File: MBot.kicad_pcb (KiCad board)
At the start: 4 copper layers, 50 x 55 mm, 111 parts, among them J1 Micro_SD_Card_Det1, J10 Conn_01x04, J11 Conn_01x06, J12 Conn_01x04, J14 Conn_01x04, J16 Conn_01x06, J2 Barrel_Jack_Switch_Pin3Ring, J3 Screw_Terminal_01x02, J4 Conn_01x03, J5 Conn_01x06, J6 Conn_01x06, J7 Conn_01x06, J8 Conn_01x04, J9 Conn_01x04, SW1 SW_SPDT, SW2 SW_SPDT, SW3 SW_SPDT, SW4 SW_SPST, U1 74AUC1G19, U2 XL4015, U3 FM24W256

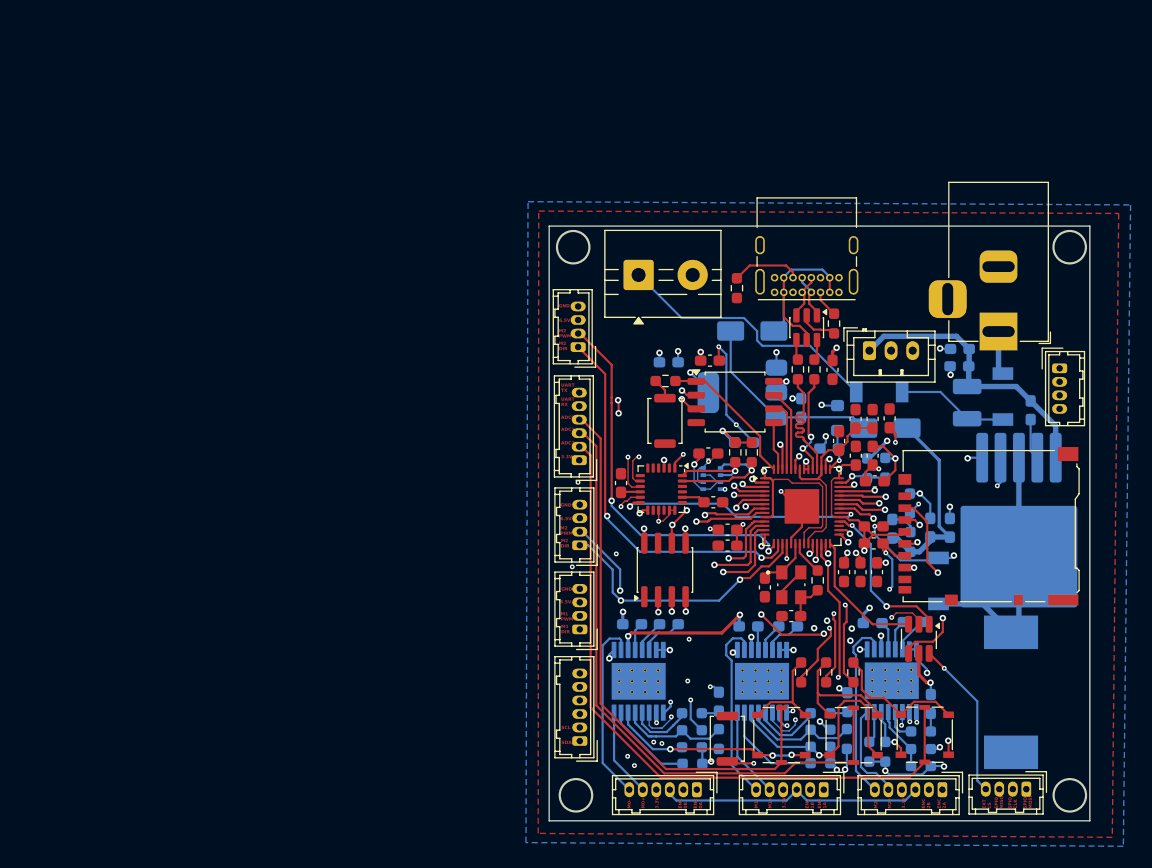
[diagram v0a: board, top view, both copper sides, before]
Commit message: Add files via upload
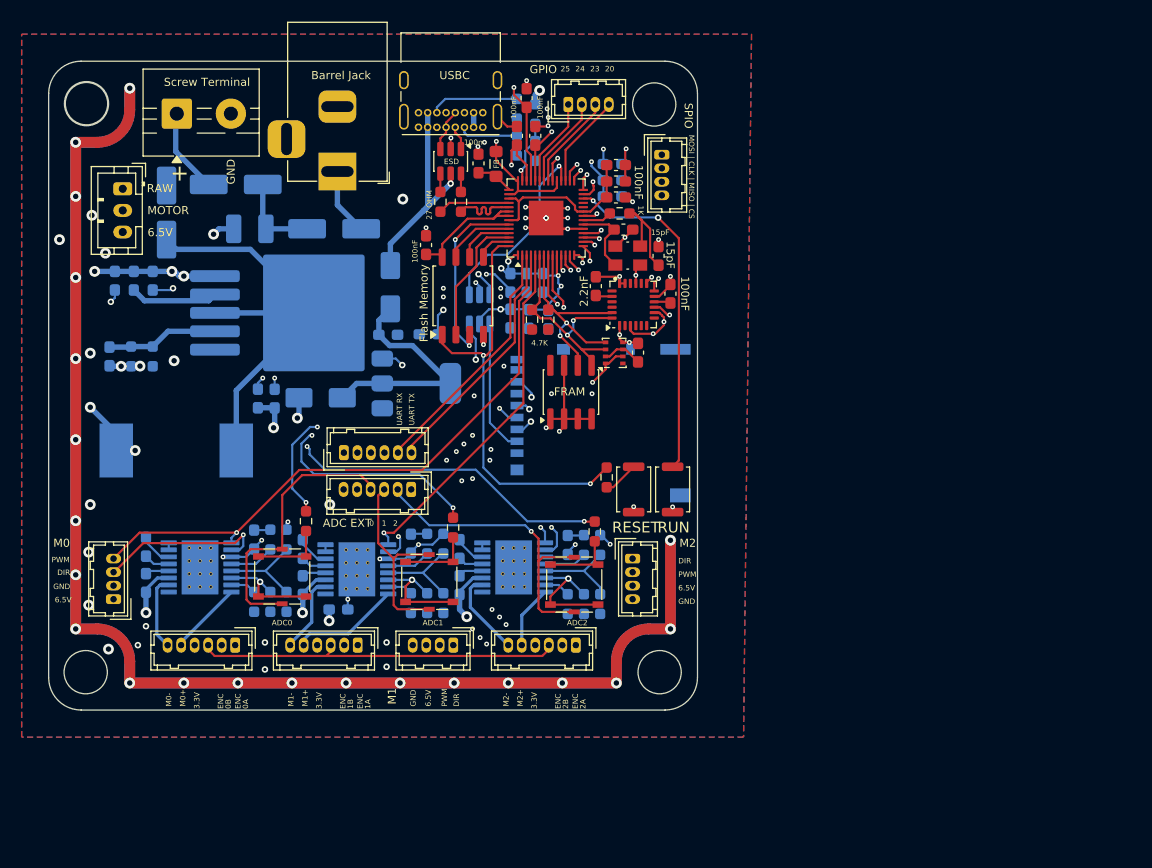
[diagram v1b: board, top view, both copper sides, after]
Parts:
- C109, C110, C111, C112, C113, C114, C115, C16, C17, J1, R109, RUSB1, U1: moved to B.Cu
- C120, FB1, UBarometer1: moved to F.Cu
- D4, D5, D6: value SS54FSH -> D; footprint SS54FSH:SODFL4725X110N -> Diode_SMD:D_SMA_Handsoldering
- moved CC1 83.8 mm to (67.9, 80.3)
- moved L1 80.4 mm to (71.8, 96.0), turned to 180 degrees
- moved D6 79.1 mm to (70.9, 74.0)
- moved C1 78.4 mm to (66.1, 80.3), turned to -90 degrees
- moved Cin1 75.0 mm to (69.6, 80.3), turned to -90 degrees
- moved CFF1 74.1 mm to (65.6, 87.3)
- moved R902 74.1 mm to (67.6, 87.3)
- moved R901 71.3 mm to (69.6, 87.3), turned to -90 degrees
- moved J4 70.7 mm to (66.8, 71.8), turned to -90 degrees
- moved U2 69.9 mm to (83.0, 83.3), turned to 0 degrees
- moved F1 68.3 mm to (78.6, 75.5), turned to 0 degrees
- moved J14 67.7 mm to (116.7, 68.7), turned to -90 degrees
- moved C18 65.1 mm to (79.3, 91.2)
- moved D4 63.8 mm to (86.4, 75.5), turned to 0 degrees
- moved J2 62.9 mm to (86.7, 70.2)
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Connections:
- F1 pad 2: Net-(D4-PadC) -> Net-(D4-K)
- J10 pad 1: M2_DIR -> M2_PWM
- J10 pad 2: M2_PWM -> M2_DIR
- J11 pad 5: UART0_RX -> unconnected-(J11-Pin_5-Pad5)
- J11 pad 6: UART0_TX -> unconnected-(J11-Pin_6-Pad6)
- J12 pad 1: unconnected-(J12-Pin_1-Pad1) -> GPIO25
- J12 pad 2: GPIO25 -> GPIO24
- J12 pad 3: GPIO24 -> GPIO23
- J12 pad 4: GPIO23 -> GPIO20
- J16 pad 5: unconnected-(J16-Pin_5-Pad5) -> UART0_RX
- J16 pad 6: unconnected-(J16-Pin_6-Pad6) -> UART0_TX
- J2 pad 1: Net-(D4-PadA) -> Net-(D4-A)
- J3 pad 1: Net-(J3-Pin_1) -> Net-(D5-A)
- J5 pad 1: ENC0A -> ENC0B
- J5 pad 2: ENC0B -> ENC0A
- J6 pad 1: ENC1A -> ENC1B
- J6 pad 2: ENC1B -> ENC1A
- J7 pad 1: ENC2A -> ENC2B
- J7 pad 2: ENC2B -> ENC2A
- J8 pad 1: M0_DIR -> +6V5
- J8 pad 2: M0_PWM -> GND
- J8 pad 3: +6V5 -> M0_DIR
- J8 pad 4: GND -> M0_PWM
- L1 pad 1: Net-(U2-SW) -> Net-(D6-K)
- U2 pad 3: Net-(U2-SW) -> Net-(D6-K)
- UDRV1 pad 27: GND -> (no net)
- UDRV1 pad 28: GND -> (no net)
- UDRV1 pad 29: GND -> (no net)
- ULDO1 pad 2: +3V3 -> Net-(D101-K)
- ULDO1 pad 3: Net-(D101-K) -> +3V3
- URP2040 pad 31: /RP2040/GPIO20 -> GPIO20
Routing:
- net GND: track 150.1 -> 337.6 mm, vias 46 -> 67
- net +6V5: track 18.2 -> 138.5 mm, vias 0 -> 10
- net VMOT: track 22.7 -> 126.4 mm, vias 8 -> 13
- net ADC1: track 24.8 -> 73.8 mm
- net ADC2: track 22.2 -> 69.8 mm
- net Net-(D6-K): track 0.00 -> 41.3 mm
- net ADC1_EXT: track 57.9 -> 18.4 mm
- net ADC2_EXT: track 63.9 -> 28.5 mm, vias 0 -> 1
- net ADC0: track 26.5 -> 57.1 mm
- net +3V3: track 103.2 -> 132.0 mm, vias 30 -> 39
- net /RP2040/QSPI_SS: track 13.5 -> 39.9 mm, vias 0 -> 2
- net ADC0_EXT: track 51.8 -> 25.9 mm
- net Net-(J3-Pin_1): track 25.1 -> 0.00 mm
- net Net-(U2-SW): track 24.2 -> 0.00 mm
- net M0_DIR: track 38.4 -> 61.5 mm, vias 3 -> 2
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- added copper zone on F.Cu, net +3V3
- added copper zone on In2.Cu, net +6V5
- added copper zone on In2.Cu, net BATT
- added copper zone on B.Cu, net GND
- added copper zone on In1.Cu, net GND
- removed copper zone on In1.Cu, net +3V3
- removed copper zone on B.Cu, net +6V5
- removed copper zone on F.Cu, net GND
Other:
- board size 50 x 55 mm -> 60 x 60 mm
- board text added: "+"
- board text added: "0"
- board text added: "0A"
- board text added: "0B"
- board text added: "1"
- board text added: "100n"
- board text added: "100nF"
- board text added: "10K"
- board text added: "10uF"
- board text added: "15pF"
- board text added: "1A"
- board text added: "1B"
- board text added: "1K"
- board text added: "1uF"
- board text added: "2"
- board text added: "2.2nF"
- board text added: "20"
- board text added: "20k"
- board text added: "220"
- board text added: "220nF"
- board text added: "220uF"
- board text added: "22nF"
- board text added: "23"
- board text added: "24"
- board text added: "25"
- board text added: "27 OHM"
- board text added: "2A"
- board text added: "2B"
- board text added: "330uF"
- board text added: "33nF"
- board text added: "4.7K"
- board text added: "42K"
- board text added: "47K"
- board text added: "47uH / 5A"
- board text added: "5.1K"
- board text added: "5A"
- board text added: "74AUC1G19"
- board text added: "ADC EXT"
- board text added: "Barrel Jack"
- board text added: "DIR"
- board text added: "ENC"
- board text added: "ESD"
- board text added: "FB"
- board text added: "FRAM"
- board text added: "FUSE"
- board text added: "Flash Memory"
- board text added: "GPIO"
- board text added: "LED"
- board text added: "M0"
- board text added: "M1"
- board text added: "M2"
- board text added: "MOSI | CLK | MISO | CS"
- board text added: "MOTOR"
- board text added: "NCP1117"
- board text added: "PWM"
- board text added: "RAW"
- board text added: "RESET"
- board text added: "RUN"
- board text added: "SPIO"
- board text added: "SS14"
- board text added: "SS54"
- board text added: "Screw Terminal"
- board text added: "USBC"
- board text added: "XL4015"
- board text removed: "ENC 0A"
- board text removed: "ENC 0B"
- board text removed: "ENC 1A"
- board text removed: "ENC 1B"
- board text removed: "ENC 2A"
- board text removed: "ENC 2B"
- board text removed: "EXT CS"
- board text removed: "M1 DIR"
- board text removed: "M1 PWM"
- board text removed: "M2 DIR"
- board text removed: "M2 PWM"
- board text removed: "SCL"
- board text removed: "SDA"
- board text removed: "SPIO CLK"
- board text removed: "SPIO MISO"
- board text removed: "SPIO MOSI"
